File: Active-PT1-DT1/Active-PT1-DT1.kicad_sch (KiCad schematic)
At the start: 27 parts, among them U1 Opamp_Dual

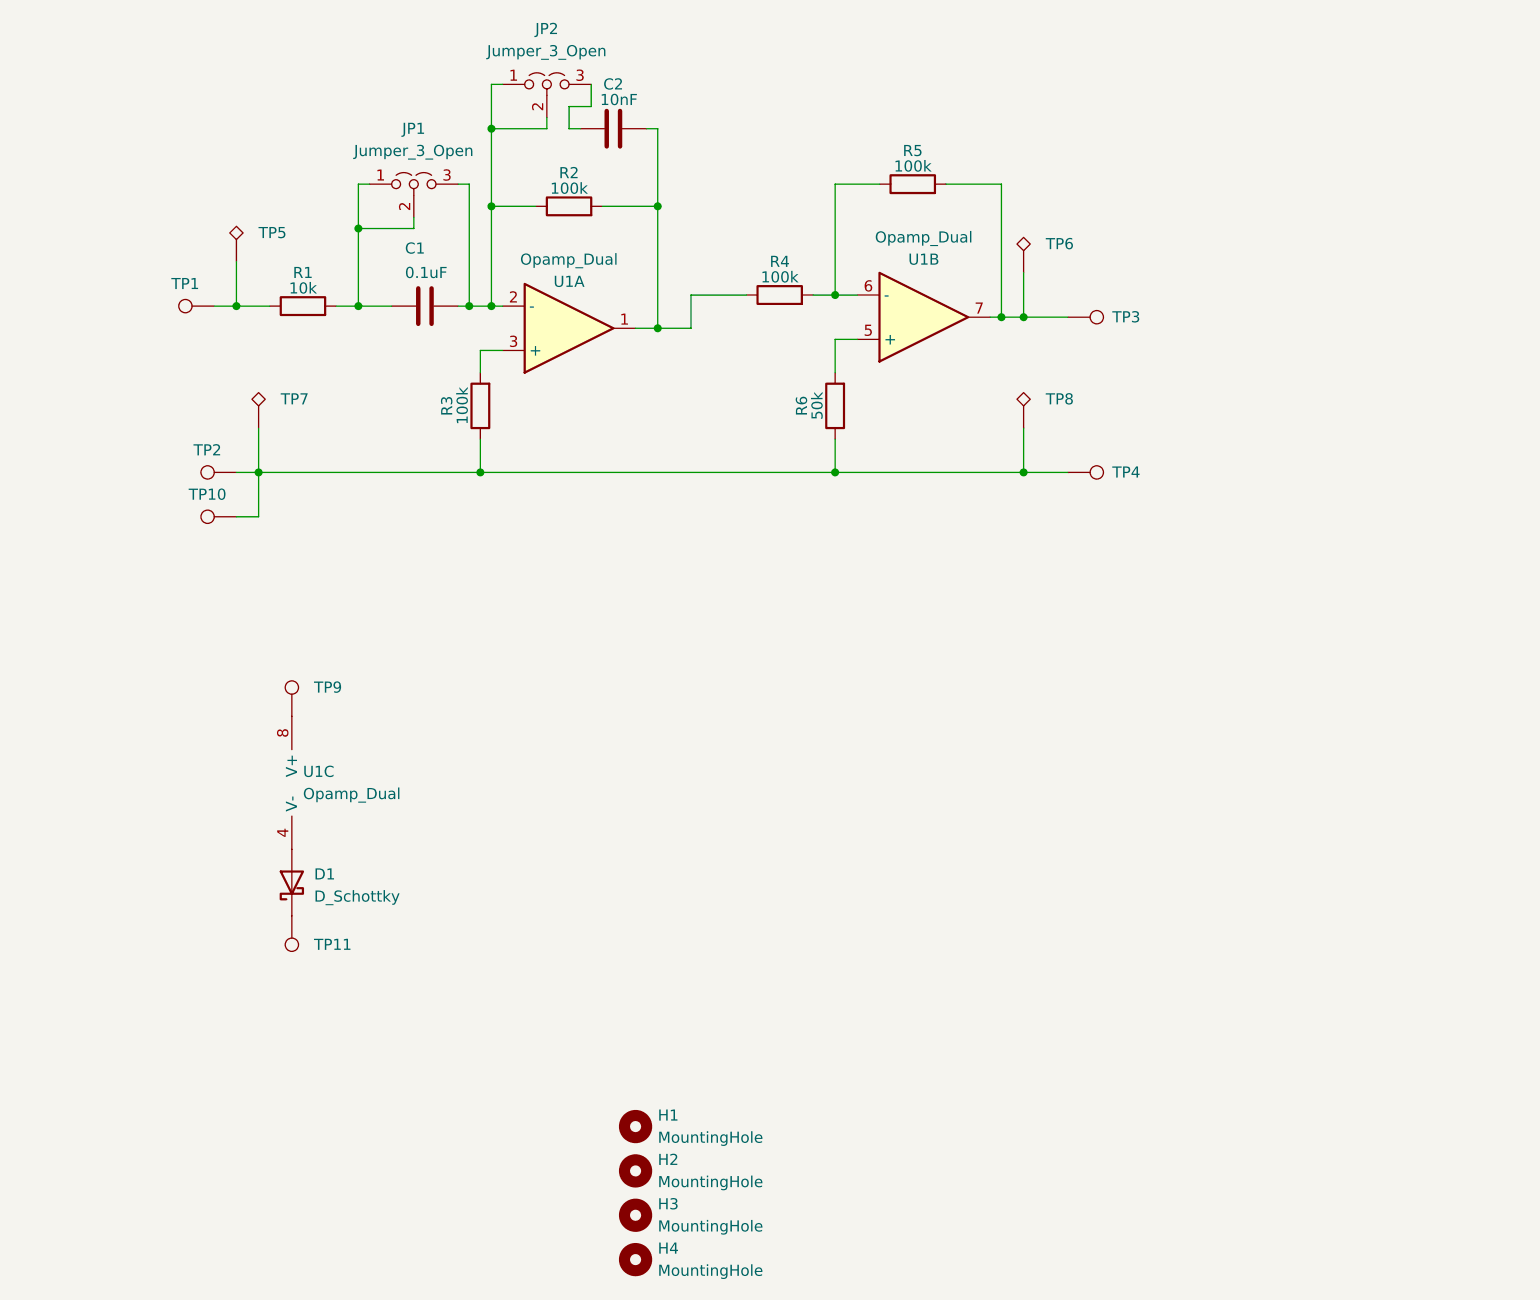
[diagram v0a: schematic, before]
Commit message: PT1/DT1/P
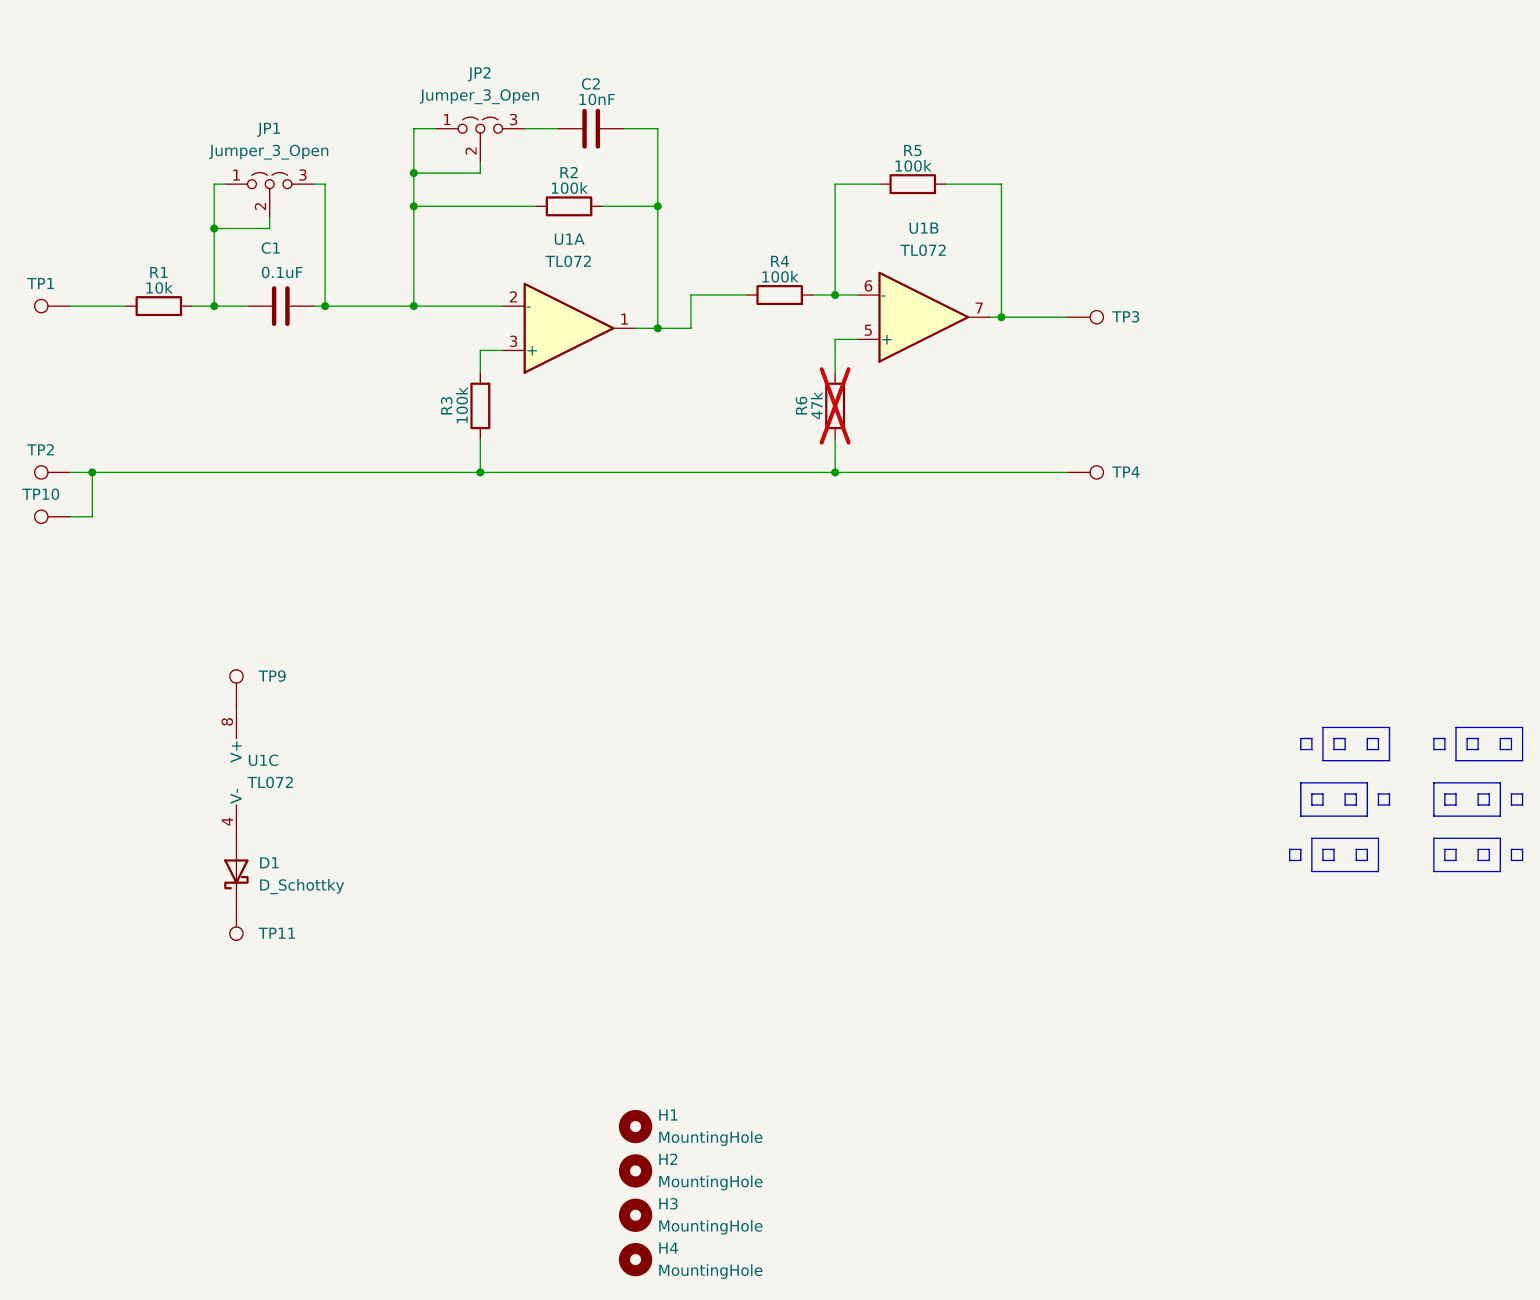
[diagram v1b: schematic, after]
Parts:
- removed TP5, TP6, TP7, TP8: TestPoint_Alt, Library:KEYS4952, symbol Connector:TestPoint_Alt
- removed U1: Opamp_Dual, Package_DIP:DIP-8_W7.62mm_Socket_LongPads, symbol Device:Opamp_Dual
- added U1: TL072, Package_DIP:DIP-8_W7.62mm_LongPads, symbol Amplifier_Operational:TL072
- C1, C2: footprint Capacitor_THT:C_Rect_L7.2mm_W5.0mm_P5.00mm -> (none)
- R6: value 50k -> 47k; now not fitted
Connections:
- net at C1.2, JP1.3 (B), JP2.1 (A)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: now also U1.2 (-)
- net at C2.2, R2.2, R4.1: now also U1.1
- net at TP9.1: now also U1.8 (V+)
- net at R6.2: now also U1.5 (+)
- net at R5.2, TP3.1: now also U1.7
- net at R4.2, R5.1: now also U1.6 (-)
- net at R3.2: now also U1.3 (+)
- net at D1.2 (A): now also U1.4 (V-)
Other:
- moved on the sheet: C1, C2, D1, JP1, JP2, R1, TP1, TP10, TP11, TP2, TP9
